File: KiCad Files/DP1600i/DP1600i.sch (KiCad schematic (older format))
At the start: 7 parts, among them J3 Conn_01x07, J4 Conn_01x08, J5 Conn_01x04, J6 Conn_01x02, J7 Conn_02x04_Odd_Even, J8 Conn_01x05, J9 Conn_01x08

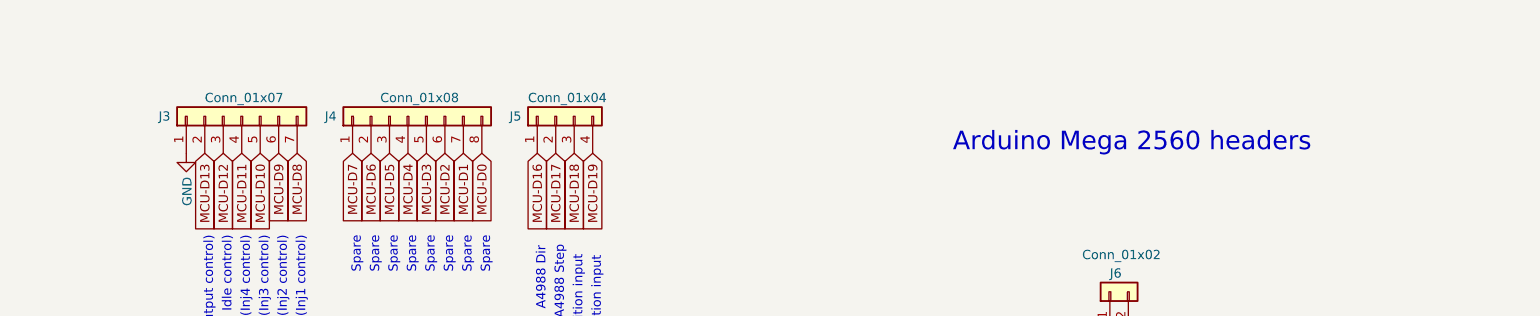
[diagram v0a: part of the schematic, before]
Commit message: Add files via upload
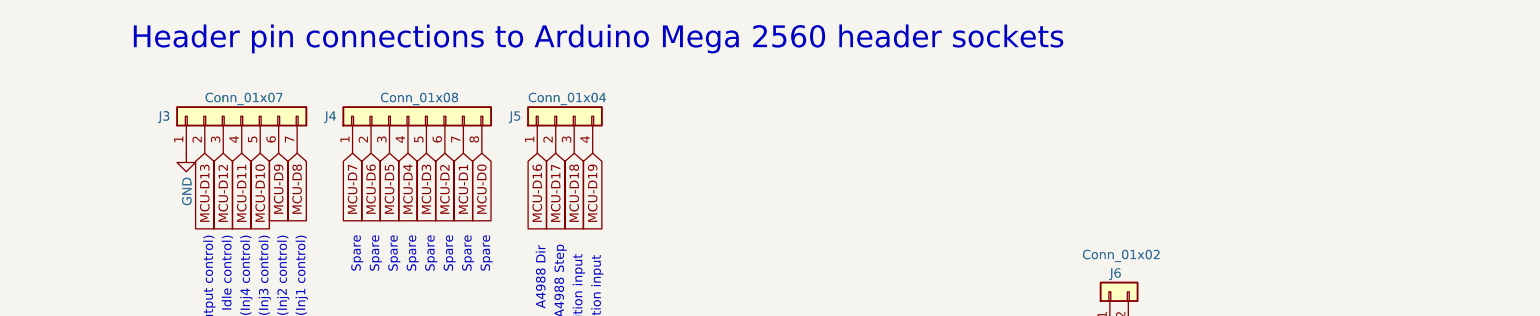
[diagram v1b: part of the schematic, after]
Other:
- note added: "Header pin connections to Arduino Mega 2560 header sockets"
- note removed: "Arduino Mega 2560 headers"
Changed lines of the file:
@@
 Text Notes 3400 1850 3    50   ~ 0
 (Inj4 control)
-Text Notes 7200 1400 0    100  ~ 0
-Arduino Mega 2560 headers
+Text Notes 2750 850  0    118  ~ 0
+Header pin connections to Arduino Mega 2560 header sockets
 Text GLabel 5250 1400 3    50   Input ~ 0
 MCU-D19
